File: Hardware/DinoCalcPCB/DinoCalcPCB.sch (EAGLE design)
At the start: 6 parts, among them U1 ATMEGA328P_PDIP

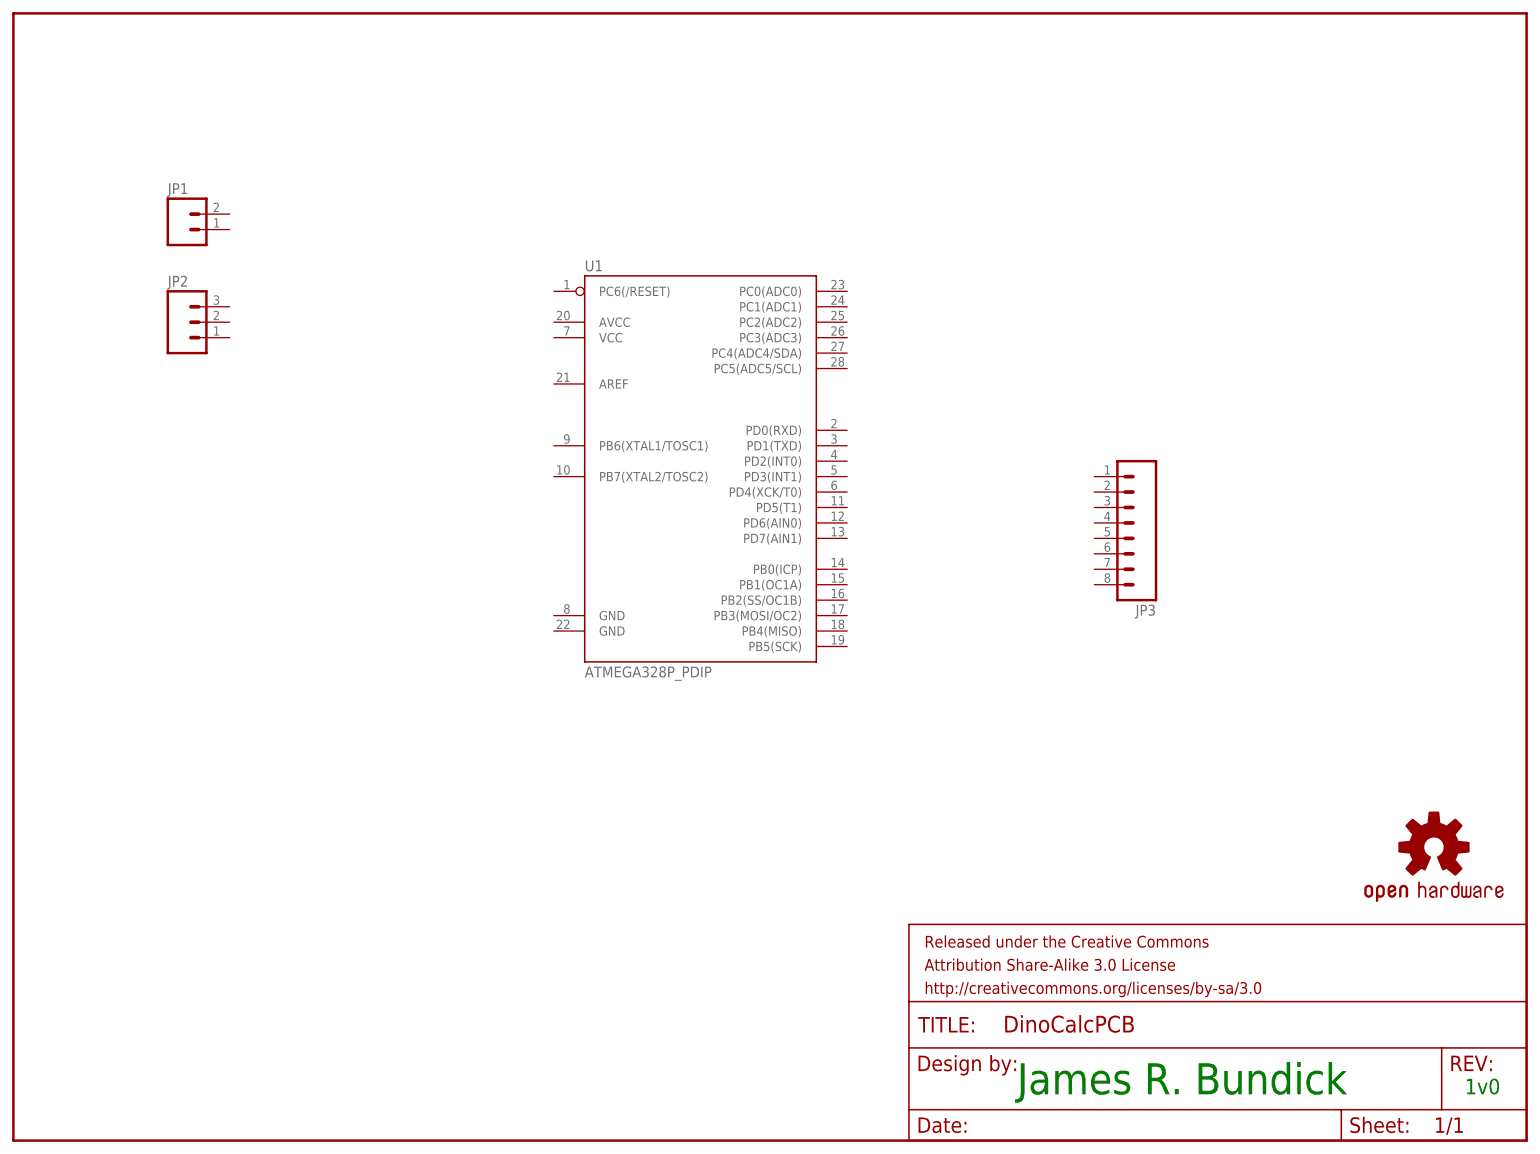
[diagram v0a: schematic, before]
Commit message: update
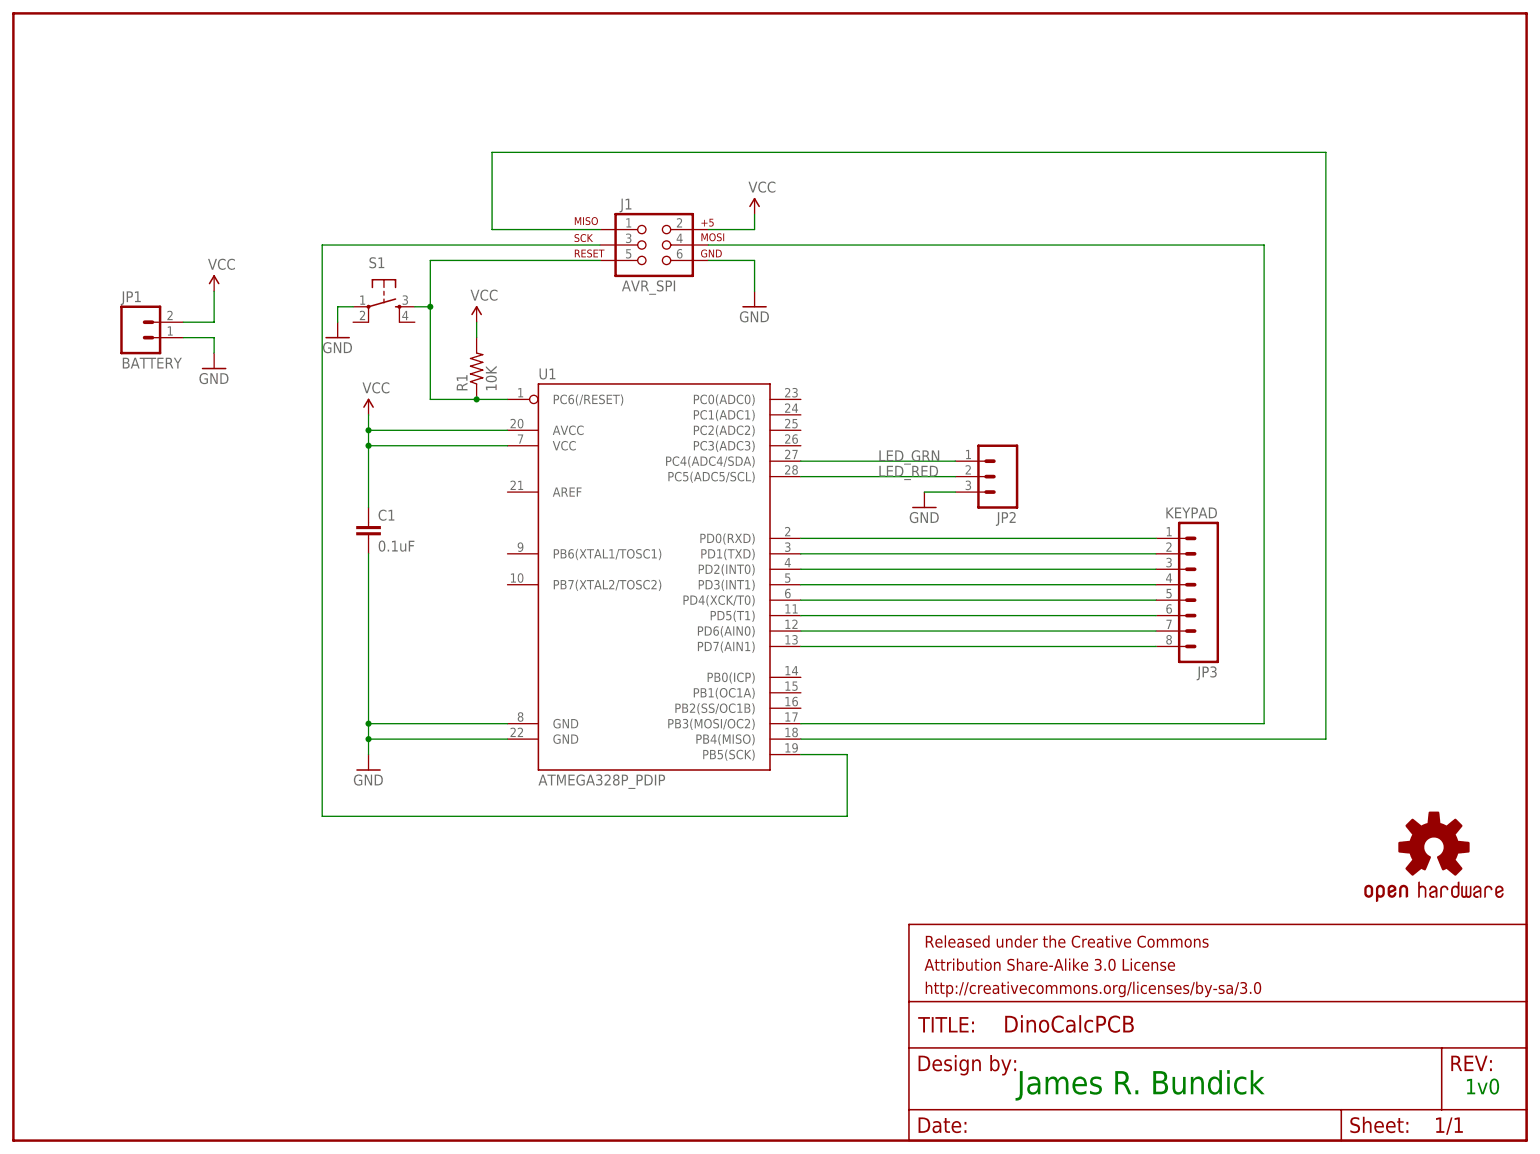
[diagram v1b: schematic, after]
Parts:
- added C1: 0.1uF, SparkFun-Capacitors:CAPPTH
- added J1: AVR_SPI, SparkFun-Connectors:AVR_SPI_PRG_6OFFSET_PADS
- added R1: 10K, SparkFun-Resistors:RESISTORPTH-1/4W
- added S1: (no value), SparkFun-Electromechanical:TAC_SWITCHPTH
- JP1: value (none) -> BATTERY
- JP3: value (none) -> KEYPAD
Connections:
- new net GND: C1.2, J1.6, JP1.1, JP2.3, S1.1, U1.GND@1, U1.GND@2
- new net LED_GRN: JP2.1, U1.PC4(ADC4/SDA)
- new net LED_RED: JP2.2, U1.PC5(ADC5/SCL)
- new net N$1: JP3.1, U1.PD0(RXD)
- new net N$10: J1.1, U1.PB4(MISO)
- new net N$13: J1.5, R1.1, S1.3, U1.PC6(/RESET)
- new net N$14: J1.3, U1.PB5(SCK)
- new net N$2: JP3.2, U1.PD1(TXD)
- new net N$3: JP3.3, U1.PD2(INT0)
- new net N$4: JP3.4, U1.PD3(INT1)
- new net N$5: JP3.5, U1.PD4(XCK/T0)
- new net N$6: JP3.6, U1.PD5(T1)
- new net N$7: JP3.7, U1.PD6(AIN0)
- new net N$8: JP3.8, U1.PD7(AIN1)
- new net N$9: J1.4, U1.PB3(MOSI/OC2)
- new net VCC: C1.1, J1.2, JP1.2, R1.2, U1.AVCC, U1.VCC
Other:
- moved on the sheet: JP1, JP2, JP3, U1
